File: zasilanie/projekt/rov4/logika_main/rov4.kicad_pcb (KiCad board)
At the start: 2 copper layers, 188 x 120 mm, 67 parts, among them IC1 UWE-12_10-Q12PB-C, J1 Battery digital, J10 Router, J11 Switch, J12 Enko_inkrementalny, J13 Torpedy, hall, laser, J14 Enko_absolutny_1, J15 Enko_absolutny_2, J16 RC_D_12V, J17 Xavier, J18 Kamera 1, J19 Kamera 2, J2 Reed switch, J20 Extra, J21 Extra, J22 hydrofony, J23 RC_D_15V, J3 RC_D_5V, J4 Manip_SterSil2, J5 Manip_SterSil1, J55 LP_OUT, J6 Extra, J7 Extra, J8 STM32, J9 RPi, Q1 IPT004N03L, Q2 IPT004N03L, Q3 BC847A, Q4 BC847A, Q5 BC847A

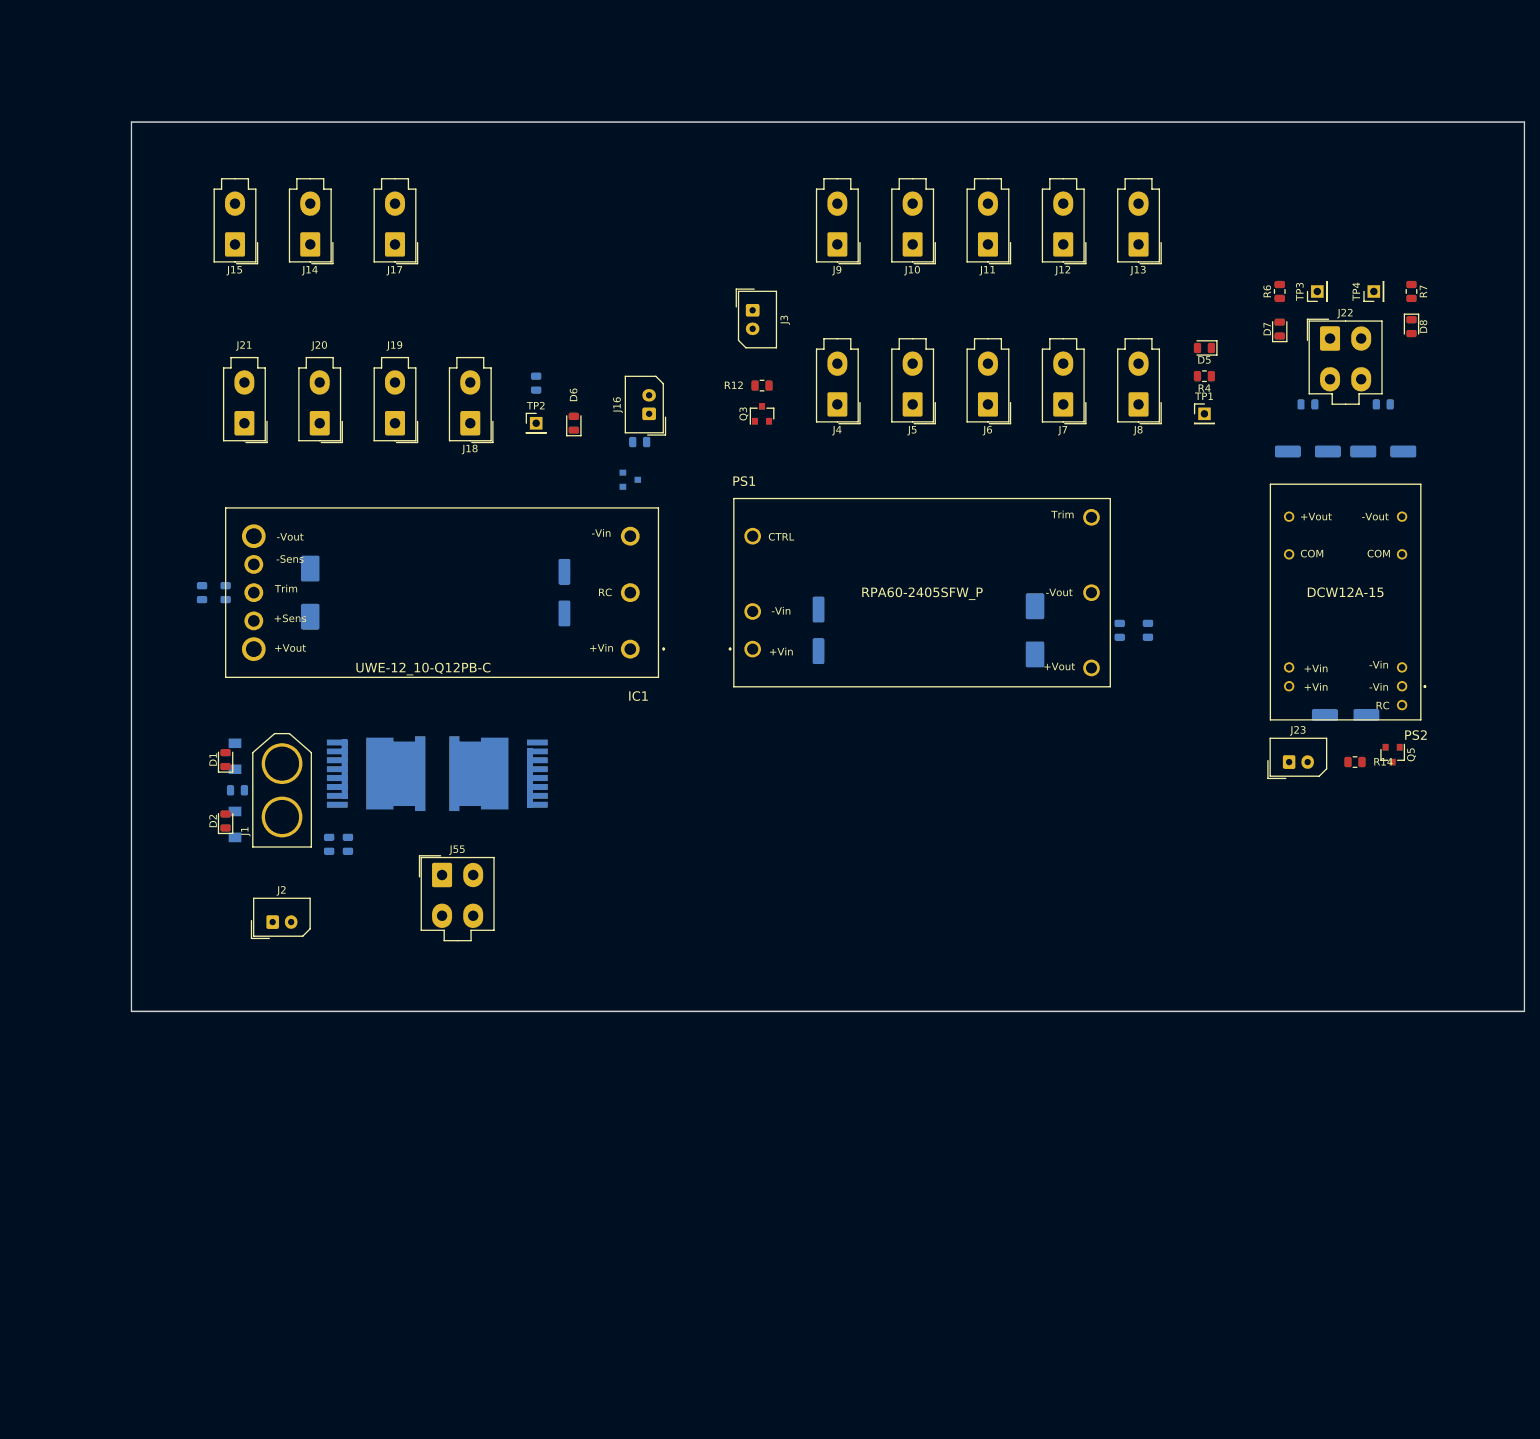
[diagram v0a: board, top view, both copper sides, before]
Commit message: Jakieś zmainy wszystkiego
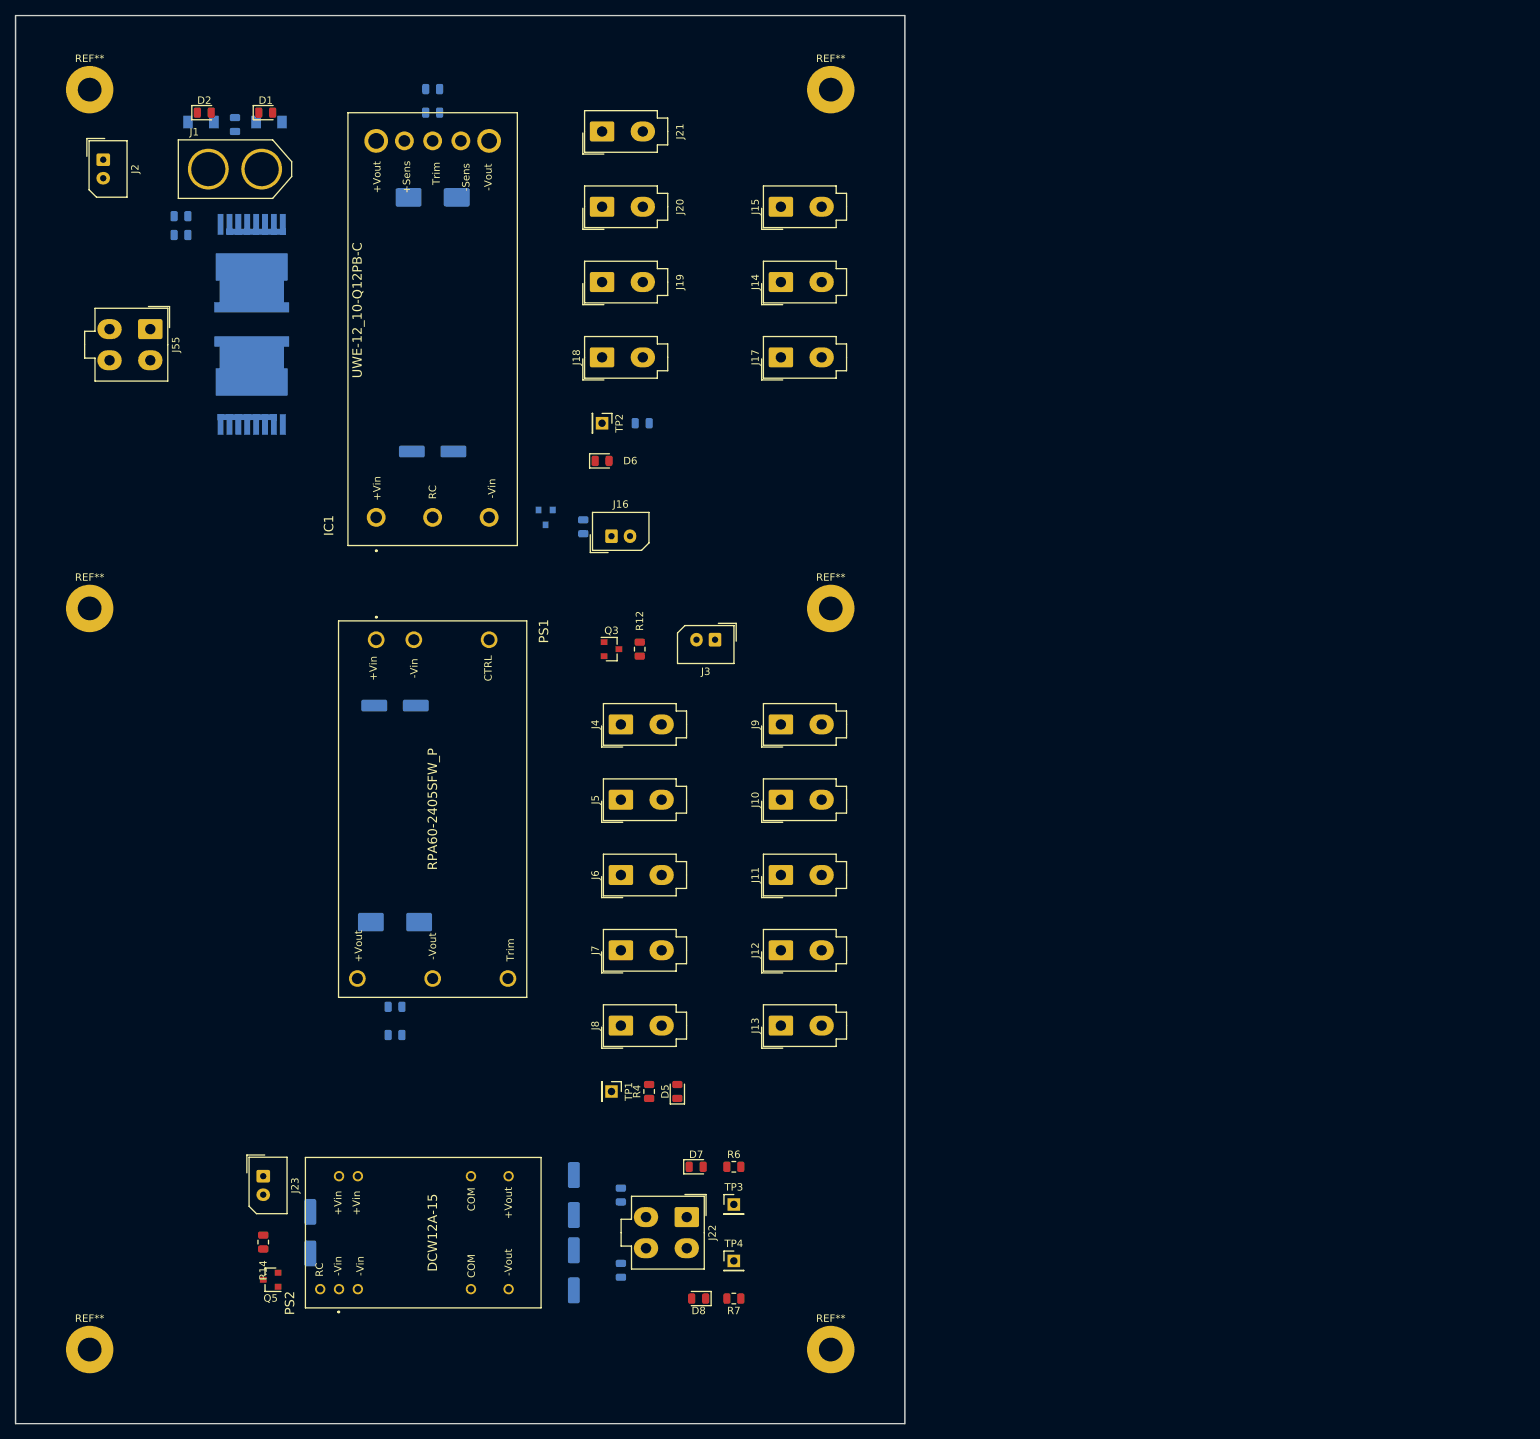
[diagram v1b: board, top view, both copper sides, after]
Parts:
- added REF**: MountingHole_3.2mm_M3_Pad, MountingHole:MountingHole_3.2mm_M3_Pad, F.Cu at (135.0, 35.0)
- added REF**: MountingHole_3.2mm_M3_Pad, MountingHole:MountingHole_3.2mm_M3_Pad, F.Cu at (35.0, 35.0)
- added REF**: MountingHole_3.2mm_M3_Pad, MountingHole:MountingHole_3.2mm_M3_Pad, F.Cu at (35.0, 105.0)
- added REF**: MountingHole_3.2mm_M3_Pad, MountingHole:MountingHole_3.2mm_M3_Pad, F.Cu at (135.0, 105.0)
- added REF**: MountingHole_3.2mm_M3_Pad, MountingHole:MountingHole_3.2mm_M3_Pad, F.Cu at (135.0, 205.0)
- added REF**: MountingHole_3.2mm_M3_Pad, MountingHole:MountingHole_3.2mm_M3_Pad, F.Cu at (35.0, 205.0)
- J10, J11, J12, J13, J14, J15, J17, J18, J19, J20, J21, J4, J5, J6, J7, J8, J9: footprint Connector_Molex:Molex_Mini-Fit_Jr_5566-02A_2x01_P4.20mm_Vertical -> molex_3d_2pin:Molex_Mini-Fit_Jr_5566-02A_2x01_P4.20mm_Vertical
- moved Q5 167.2 mm to (59.4, 195.6), turned to 180 degrees
- moved R7 163.8 mm to (121.9, 198.1), turned to 180 degrees
- moved D8 162.6 mm to (117.2, 198.1), turned to 180 degrees
- moved R14 160.9 mm to (58.4, 190.5), turned to 90 degrees
- moved TP4 156.7 mm to (121.9, 193.0), turned to 0 degrees
- moved C11 156.2 mm to (64.8, 189.2), turned to 270 degrees
- moved C12 155.7 mm to (106.7, 194.3), turned to 270 degrees
- moved C13 155.4 mm to (100.3, 194.3), turned to 270 degrees
- moved PS2 150.8 mm to (80.0, 189.2), turned to 90 degrees
- moved J23 149.3 mm to (58.4, 181.6), turned to 270 degrees
- moved J22 146.9 mm to (115.6, 187.1), turned to 270 degrees
- moved TP3 146.2 mm to (121.9, 185.4), turned to 0 degrees
- moved C9 141.3 mm to (106.7, 184.2), turned to 270 degrees
- moved C10 141.0 mm to (100.3, 184.2), turned to 270 degrees
- moved R6 139.2 mm to (121.9, 180.3), turned to 0 degrees
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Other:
- board size 188 x 120 mm -> 120 x 190 mm
- board text added: "logika main pcb"
